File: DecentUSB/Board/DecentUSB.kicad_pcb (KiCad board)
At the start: 2 copper layers, 107 x 50.9 mm, 20 parts, among them J1 USB_A_Stacked, J2 Conn_01x28_Pin, J3 Conn_02x07_Counter_Clockwise, Q1 2N7000, Q2 2N7000, Q3 TP0610L, SW1 SW_Option, U1 Pico, U2 74LS245, U5 MCP23017_SP

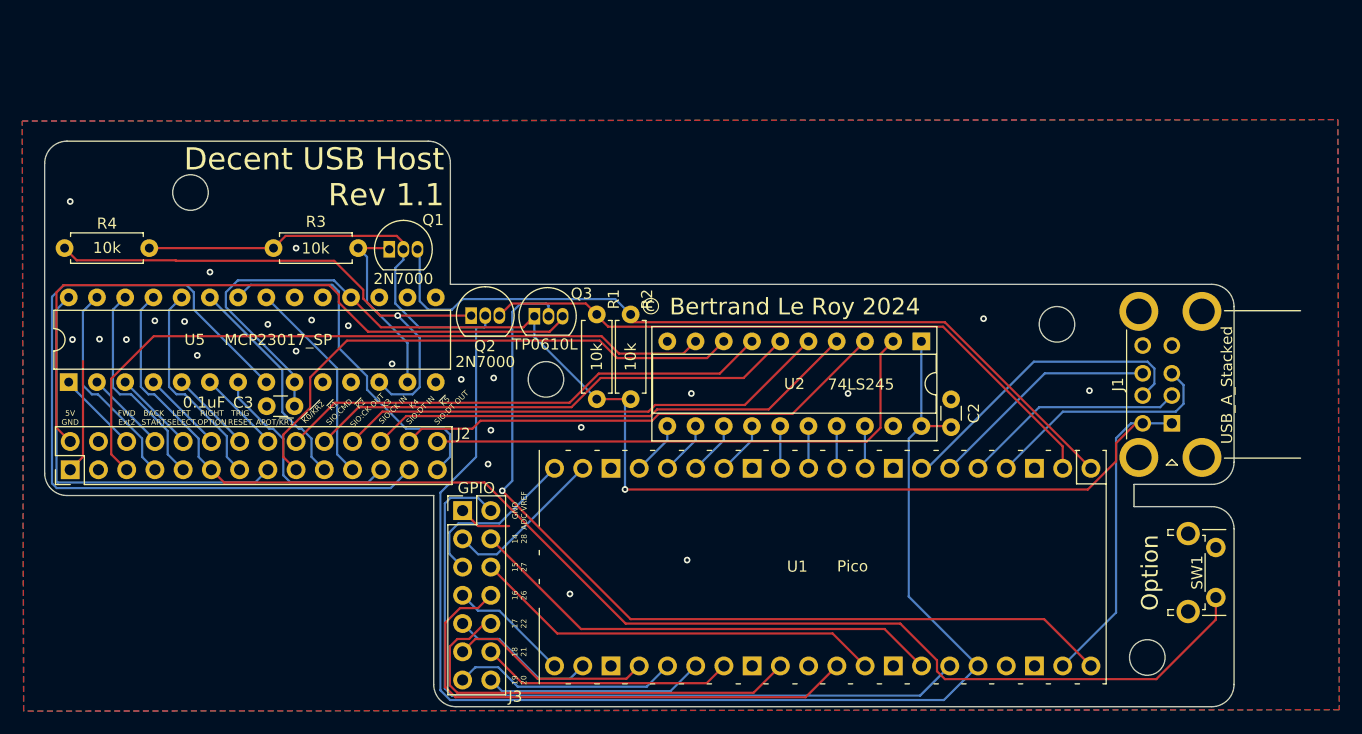
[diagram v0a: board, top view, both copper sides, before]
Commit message: DecentUSB Host board rev. 2
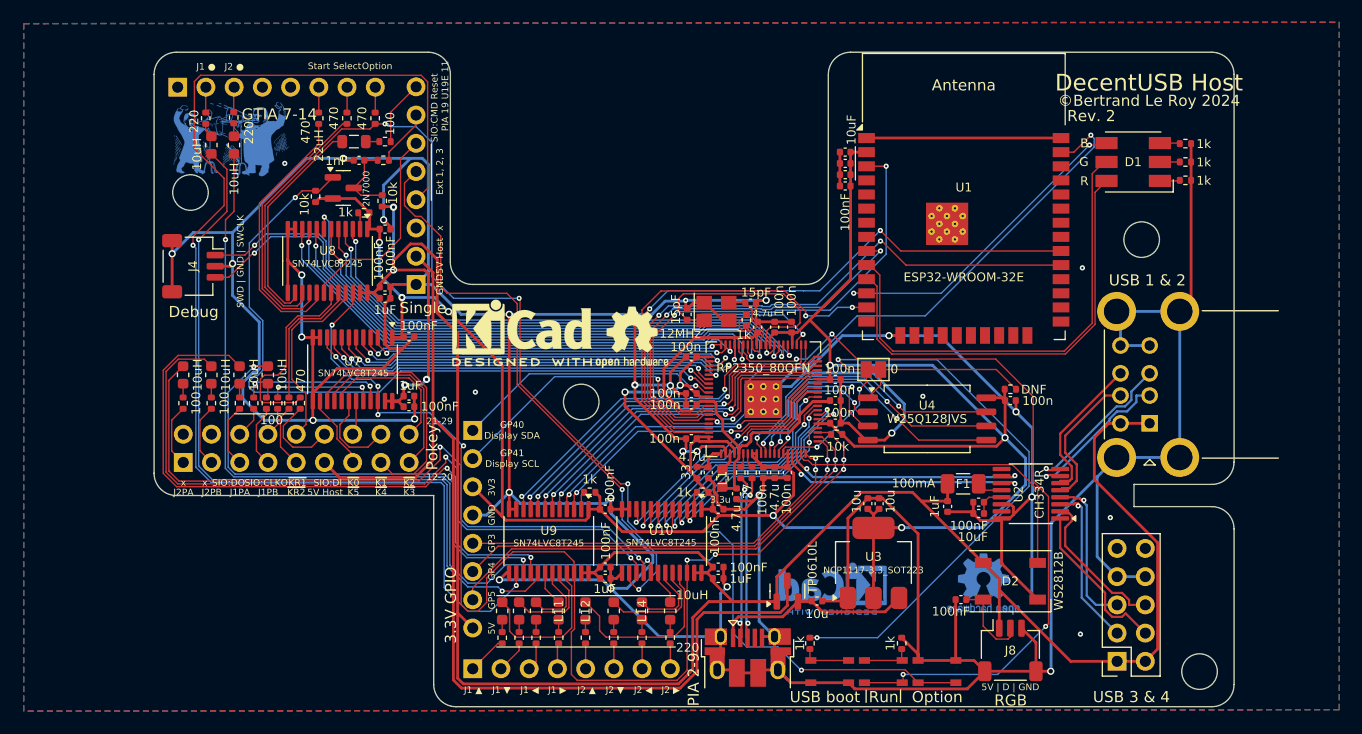
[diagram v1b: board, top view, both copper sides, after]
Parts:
- removed Q3: TP0610L, Package_TO_SOT_THT:TO-92L_Inline
- added C1: 100nF, Capacitor_SMD:C_0402_1005Metric, F.Cu at (138.4, 115.4)
- added C10: 100n, Capacitor_SMD:C_0402_1005Metric, F.Cu at (153.7, 93.9)
- added C11: 100n, Capacitor_SMD:C_0402_1005Metric, F.Cu at (146.2, 103.9)
- added C12: 100n, Capacitor_SMD:C_0402_1005Metric, F.Cu at (159.1, 102.5)
- added C13: 100n, Capacitor_SMD:C_0402_1005Metric, F.Cu at (154.8, 106.9)
- added C14: 100n, Capacitor_SMD:C_0402_1005Metric, F.Cu at (152.7, 106.9)
- added C15: 100n, Capacitor_SMD:C_0402_1005Metric, F.Cu at (155.2, 93.9)
- added C16: 100n, Capacitor_SMD:C_0402_1005Metric, F.Cu at (146.2, 96.5)
- added C17: 100n, Capacitor_SMD:C_0402_1005Metric, F.Cu at (146.2, 99.8)
- added C18: 4.7u, Capacitor_SMD:C_0402_1005Metric, F.Cu at (147.7, 106.9)
- added C19: 4.7u, Capacitor_SMD:C_0402_1005Metric, F.Cu at (153.7, 106.9)
- added C20: 4.7u, Capacitor_SMD:C_0402_1005Metric, F.Cu at (150.2, 108.8)
- added C21: 100n, Capacitor_SMD:C_0402_1005Metric, F.Cu at (174.9, 100.5)
- added C22: 10u, Capacitor_SMD:C_0402_1005Metric, F.Cu at (163.1, 109.7)
- added C23: 1nF, Capacitor_SMD:C_0402_1005Metric, F.Cu at (116.3, 78.8)
- added C24: 100nF, Capacitor_SMD:C_0402_1005Metric, F.Cu at (172.0, 109.6)
- added C25: 1uF, Capacitor_SMD:C_0402_1005Metric, F.Cu at (169.2, 110.0)
- added C26: 1uF, Capacitor_SMD:C_0402_1005Metric, F.Cu at (138.4, 116.5)
- added C27: 100nF, Capacitor_SMD:C_0402_1005Metric, F.Cu at (120.8, 101.0)
- added C28: 1uF, Capacitor_SMD:C_0402_1005Metric, F.Cu at (120.8, 100.1)
- added C29: 100nF, Capacitor_SMD:C_0402_1005Metric, F.Cu at (118.6, 90.2)
- added C30: 1uF, Capacitor_SMD:C_0402_1005Metric, F.Cu at (118.6, 91.3)
- added C31: 15pF, Capacitor_SMD:C_0402_1005Metric, F.Cu at (151.5, 91.7)
- added C32: 100nF, Capacitor_SMD:C_0402_1005Metric, F.Cu at (148.6, 115.4)
- added C33: 1uF, Capacitor_SMD:C_0402_1005Metric, F.Cu at (148.6, 116.5)
- added C34: 100nF, Capacitor_SMD:C_0402_1005Metric, F.Cu at (120.8, 94.7)
- added C35: 100nF, Capacitor_SMD:C_0402_1005Metric, F.Cu at (118.6, 85.0)
- added C36: 100nF, Capacitor_SMD:C_0402_1005Metric, F.Cu at (138.4, 110.2)
- added C37: 100nF, Capacitor_SMD:C_0402_1005Metric, F.Cu at (148.6, 110.2)
- added C38: 10uF, Capacitor_SMD:C_0402_1005Metric, F.Cu at (160.0, 78.1)
- added C39: 10uF, Capacitor_SMD:C_0402_1005Metric, F.Cu at (160.0, 79.1)
- added C4: 10u, Capacitor_SMD:C_0402_1005Metric, F.Cu at (157.5, 118.5)
- added C40: 10uF, Capacitor_SMD:C_0402_1005Metric, F.Cu at (160.0, 80.1)
- added C41: 100nF, Capacitor_SMD:C_0402_1005Metric, F.Cu at (160.0, 81.2)
- added C42: 100nF, Capacitor_SMD:C_0402_1005Metric, F.Cu at (170.4, 118.4)
- added C5: 10u, Capacitor_SMD:C_0402_1005Metric, F.Cu at (162.1, 109.7)
- added C6: 100n, Capacitor_SMD:C_0402_1005Metric, F.Cu at (146.2, 100.8)
- added C7: 4.7u, Capacitor_SMD:C_0402_1005Metric, F.Cu at (152.1, 93.9)
- added C8: 100n, Capacitor_SMD:C_0402_1005Metric, F.Cu at (159.1, 100.5)
- added C9: 100n, Capacitor_SMD:C_0402_1005Metric, F.Cu at (159.1, 98.6)
- added D1: LED_RGB, LED_SMD:LED_RGB_5050-6, F.Cu at (185.9, 79.0)
- added D2: WS2812B, LED_SMD:LED_WS2812B_PLCC4_5.0x5.0mm_P3.2mm, F.Cu at (174.9, 116.7)
- added F1: 100mA, Fuse:Fuse_1206_3216Metric, F.Cu at (170.6, 108.0)
- added G***: LOGO, Library:ScreamingAtTheRadio, B.Cu at (104.6, 75.9)
- added J1: USB_B_Micro, Connector_USB:USB_Micro-B_Amphenol_10103594-0001LF_Horizontal, F.Cu at (151.3, 123.6)
- added J4: SM03B-SRSS-TB, Connector_JST:JST_SH_SM03B-SRSS-TB_1x03-1MP_P1.00mm_Horizontal, F.Cu at (101.3, 88.4)
- added J5: Conn_02x09_Counter_Clockwise, Connector_PinSocket_2.54mm:PinSocket_2x09_P2.54mm_Vertical, F.Cu at (100.5, 103.5)
- added J6: Conn_02x05_Odd_Even, Connector_PinSocket_2.54mm:PinSocket_2x05_P2.54mm_Vertical, F.Cu at (184.5, 123.9)
- added J7: Conn_01x08, Connector_PinHeader_2.54mm:PinHeader_1x08_P2.54mm_Vertical, F.Cu at (126.5, 124.6)
- added J8: Conn_01x03, Connector_JST:JST_SH_SM03B-SRSS-TB_1x03-1MP_P1.00mm_Horizontal, F.Cu at (174.9, 122.9)
- added J9: Conn_01x08, Connector_PinHeader_2.54mm:PinHeader_1x08_P2.54mm_Vertical, F.Cu at (126.5, 103.1)
- added L1: 3.3u, Inductor_SMD:L_0603_1608Metric, F.Cu at (149.0, 107.4)
- added L10: 10uH, Inductor_SMD:L_0603_1608Metric, F.Cu at (132.2, 119.4)
- added L11: 10uH, Inductor_SMD:L_0603_1608Metric, F.Cu at (134.2, 119.4)
- added L12: 10uH, Inductor_SMD:L_0603_1608Metric, F.Cu at (136.7, 119.4)
- added L13: 10uH, Inductor_SMD:L_0603_1608Metric, F.Cu at (139.2, 119.4)
- added L14: 10uH, Inductor_SMD:L_0603_1608Metric, F.Cu at (141.7, 119.4)
- added L15: 10uH, Inductor_SMD:L_0603_1608Metric, F.Cu at (144.3, 119.4)
- added L16: 22uH, Inductor_SMD:L_0805_2012Metric, F.Cu at (115.8, 77.2)
- added L2: 10uH, Inductor_SMD:L_0603_1608Metric, F.Cu at (100.5, 98.2)
- added L3: 10uH, Inductor_SMD:L_0603_1608Metric, F.Cu at (103.0, 98.2)
- added L4: 10uH, Inductor_SMD:L_0603_1608Metric, F.Cu at (105.5, 98.2)
- added L5: 10uH, Inductor_SMD:L_0603_1608Metric, F.Cu at (108.1, 98.2)
- added L6: 10uH, Inductor_SMD:L_0603_1608Metric, F.Cu at (103.0, 77.5)
- added L7: 10uH, Inductor_SMD:L_0603_1608Metric, F.Cu at (105.0, 77.5)
- added L8: 10uH, Inductor_SMD:L_0603_1608Metric, F.Cu at (129.2, 119.4)
- added L9: 10uH, Inductor_SMD:L_0603_1608Metric, F.Cu at (130.7, 119.4)
- added R12: 10k, Resistor_SMD:R_0402_1005Metric, F.Cu at (112.4, 82.1)
- added R13: 10k, Resistor_SMD:R_0402_1005Metric, F.Cu at (118.4, 82.5)
- added R14: 100, Resistor_SMD:R_0402_1005Metric, F.Cu at (109.0, 100.7)
- added R15: 100, Resistor_SMD:R_0402_1005Metric, F.Cu at (106.8, 100.7)
- added R16: 100, Resistor_SMD:R_0402_1005Metric, F.Cu at (111.0, 100.7)
- added R17: 100, Resistor_SMD:R_0402_1005Metric, F.Cu at (100.5, 100.7)
- added R18: 100, Resistor_SMD:R_0402_1005Metric, F.Cu at (103.0, 100.7)
- added R19: 100, Resistor_SMD:R_0402_1005Metric, F.Cu at (105.5, 100.7)
- added R20: 100, Resistor_SMD:R_0402_1005Metric, F.Cu at (107.9, 100.7)
- added R21: 470, Resistor_SMD:R_0402_1005Metric, F.Cu at (110.0, 100.7)
- added R22: 220, Resistor_SMD:R_0402_1005Metric, F.Cu at (102.5, 75.1)
- added R23: 220, Resistor_SMD:R_0402_1005Metric, F.Cu at (105.0, 75.0)
- added R24: 470, Resistor_SMD:R_0402_1005Metric, F.Cu at (112.6, 75.1)
- added R25: 470, Resistor_SMD:R_0402_1005Metric, F.Cu at (115.2, 75.1)
- added R26: 470, Resistor_SMD:R_0402_1005Metric, F.Cu at (117.7, 75.1)
- added R27: 220, Resistor_SMD:R_0402_1005Metric, F.Cu at (129.2, 121.8)
- added R28: 220, Resistor_SMD:R_0402_1005Metric, F.Cu at (130.7, 121.8)
- added R29: 220, Resistor_SMD:R_0402_1005Metric, F.Cu at (132.2, 121.8)
- added R30: 220, Resistor_SMD:R_0402_1005Metric, F.Cu at (134.2, 121.8)
- added R31: 220, Resistor_SMD:R_0402_1005Metric, F.Cu at (136.7, 121.8)
- added R32: 220, Resistor_SMD:R_0402_1005Metric, F.Cu at (139.2, 121.8)
- added R33: 220, Resistor_SMD:R_0402_1005Metric, F.Cu at (141.7, 121.8)
- added R34: 220, Resistor_SMD:R_0402_1005Metric, F.Cu at (144.3, 121.8)
- added R35: 100, Resistor_SMD:R_0402_1005Metric, F.Cu at (118.6, 77.2)
- added R36: 10k, Resistor_SMD:R_0402_1005Metric, F.Cu at (159.3, 103.5)
- added R37: 1k, Resistor_SMD:R_0402_1005Metric, F.Cu at (116.7, 83.6)
- added R38: 1k, Resistor_SMD:R_0402_1005Metric, F.Cu at (137.0, 108.7)
- added R39: 1k, Resistor_SMD:R_0402_1005Metric, F.Cu at (147.2, 108.7)
- added R40: 1k, Resistor_SMD:R_0402_1005Metric, F.Cu at (190.6, 80.6)
- added R41: 1k, Resistor_SMD:R_0402_1005Metric, F.Cu at (190.6, 79.0)
- added R42: 1k, Resistor_SMD:R_0402_1005Metric, F.Cu at (190.6, 77.3)
- added R5: DNF, Resistor_SMD:R_0402_1005Metric, F.Cu at (174.9, 99.4)
- added R6: 100, Resistor_SMD:R_0402_1005Metric, F.Cu at (118.5, 78.8)
- added R7: 1k, Resistor_SMD:R_0402_1005Metric, F.Cu at (156.8, 122.3)
- added R8: 0, Jumper:SolderJumper-2_P1.3mm_Bridged_Pad1.0x1.5mm, F.Cu at (162.6, 97.7)
- added R9: 1k, Resistor_SMD:R_0402_1005Metric, F.Cu at (165.1, 122.3)
- added REF**: KiCad-Logo2_5mm_SilkScreen, Symbol:KiCad-Logo2_5mm_SilkScreen, F.Cu at (130.9, 94.4)
- added REF**: OSHW-Logo2_7.3x6mm_SilkScreen, Symbol:OSHW-Logo2_7.3x6mm_SilkScreen, F.Cu at (140.8, 94.8)
- added REF**: OSHW-Logo2_7.3x6mm_Copper, Symbol:OSHW-Logo2_7.3x6mm_Copper, B.Cu at (172.5, 117.0)
- added REF**: KiCad-Logo2_6mm_Copper, Symbol:KiCad-Logo2_6mm_Copper, B.Cu at (158.9, 116.7)
- added SW2: SW_USB_BOOT, DecenTKL:SW_Push_1P1T_XKB_TS-1177A-C, F.Cu at (158.6, 124.8)
- added SW3: SW_RUN, DecenTKL:SW_Push_1P1T_XKB_TS-1177A-C, F.Cu at (163.4, 124.8)
- added U10: SN74LVC8T245, Package_SO:TSSOP-24_4.4x7.8mm_P0.65mm, F.Cu at (143.5, 113.1)
- added U3: NCP1117-3.3_SOT223, Package_TO_SOT_SMD:SOT-223-3_TabPin2, F.Cu at (162.6, 115.1)
- added U4: W25Q128JVS, Package_SO:SOIC-8_7.5x5.85mm_P1.27mm, F.Cu at (167.4, 102.1)
- added U7: SN74LVC8T245, Package_SO:TSSOP-24_4.4x7.8mm_P0.65mm, F.Cu at (115.7, 97.6)
- added U8: SN74LVC8T245, Package_SO:TSSOP-24_4.4x7.8mm_P0.65mm, F.Cu at (113.4, 87.9)
- added U9: SN74LVC8T245, Package_SO:TSSOP-24_4.4x7.8mm_P0.65mm, F.Cu at (133.3, 113.1)
- added X4: 12MHz, Crystal:Crystal_SMD_Abracon_ABM8AIG-4Pin_3.2x2.5mm, F.Cu at (148.4, 92.4)
- C2: value 0.1uF -> 15pF; footprint Capacitor_THT:C_Disc_D3.0mm_W1.6mm_P2.50mm -> Capacitor_SMD:C_0402_1005Metric
- C3: value 0.1uF -> 10uF; footprint Capacitor_THT:C_Disc_D3.0mm_W1.6mm_P2.50mm -> Capacitor_SMD:C_0402_1005Metric
- J2: value Conn_01x28_Pin -> Conn_01x08; footprint Connector_PinHeader_2.54mm:PinHeader_2x14_P2.54mm_Vertical -> Connector_PinHeader_2.54mm:PinHeader_1x08_P2.54mm_Vertical
- J3: value Conn_02x07_Counter_Clockwise -> Conn_01x08; footprint Connector_PinHeader_2.54mm:PinHeader_2x07_P2.54mm_Vertical -> Connector_PinHeader_2.54mm:PinHeader_1x08_P2.54mm_Vertical
- Q1: footprint Package_TO_SOT_THT:TO-92_Inline -> Package_TO_SOT_SMD:SOT-23
- Q2: value 2N7000 -> TP0610L; footprint Package_TO_SOT_THT:TO-92_Inline -> Package_TO_SOT_SMD:SOT-23
- R1: value 10k -> 1k; footprint Resistor_THT:R_Axial_DIN0207_L6.3mm_D2.5mm_P7.62mm_Horizontal -> Resistor_SMD:R_0402_1005Metric
- R2: value 10k -> 33; footprint Resistor_THT:R_Axial_DIN0207_L6.3mm_D2.5mm_P7.62mm_Horizontal -> Resistor_SMD:R_0402_1005Metric
- R3, R4: value 10k -> 27; footprint Resistor_THT:R_Axial_DIN0207_L6.3mm_D2.5mm_P7.62mm_Horizontal -> Resistor_SMD:R_0402_1005Metric
- SW1: footprint Button_Switch_THT:SW_Tactile_SPST_Angled_PTS645Vx83-2LFS -> DecenTKL:SW_Push_1P1T_XKB_TS-1177A-C
- U1: value Pico -> ESP32-WROOM-32E; footprint Library:RPi_Pico_TH -> RF_Module:ESP32-WROOM-32D
- U2: value 74LS245 -> CH334R; footprint Package_DIP:DIP-20_W7.62mm_Socket -> Package_SO:QSOP-16_3.9x4.9mm_P0.635mm
- U5: value MCP23017_SP -> RP2350_80QFN; footprint Package_DIP:DIP-28_W7.62mm -> DecenTKL:RP2350-QFN-80-1EP_10x10_P0.4mm_EP3.4x3.4mm_ThermalVias
- USB1-2: renamed from J1; value USB_A_Stacked -> USB_A_Dual
- moved C3 64.8 mm to (172.0, 110.6), turned to 180 degrees
- moved U5 62.5 mm to (152.7, 100.3), turned to 180 degrees
- moved R4 56.9 mm to (150.6, 106.9), turned to 90 degrees
- moved R3 47.6 mm to (151.6, 106.9), turned to 90 degrees
- moved J3 45.9 mm to (100.0, 72.3), turned to 90 degrees
- moved Q2 37.7 mm to (154.8, 117.6), turned to 90 degrees
- moved J2 35.3 mm to (121.4, 90.0), turned to 180 degrees
- moved U1 32.9 mm to (170.7, 85.1), turned to 0 degrees
- moved SW1 27.5 mm to (168.3, 124.8), turned to 0 degrees
- moved C2 24.9 mm to (145.8, 92.7), turned to 90 degrees
- moved U2 16.9 mm to (176.7, 108.8), turned to 180 degrees
- moved R1 15.2 mm to (151.1, 93.2)
- moved REF** 10.8 mm to (186.7, 86.0)
- moved R2 8.90 mm to (146.7, 106.9)
- moved Q1 6.90 mm to (114.9, 81.3)
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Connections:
- C2 pad 1: GND -> /XIN
- C2 pad 2: 3.3V -> GND
- C3 pad 1: unconnected-(C3-Pad1) -> Net-(U2-VDD33)
- C3 pad 2: 5V -> GND
- J2 pad 2: unconnected-(J2-Pin_2-Pad2) -> +5V HOST
- J2 pad 3: EXT2 -> unconnected-(J2-Pin_3-Pad3)
- J2 pad 4: START -> EXT1
- J2 pad 5: SELECT -> EXT2
- J2 pad 6: OPTION -> EXT3
- J2 pad 7: RESET -> Net-(J2-Pin_7)
- J2 pad 8: ~{KR1} -> Net-(J2-Pin_8)
- J3 pad 1: GND -> unconnected-(J3-Pin_1-Pad1)
- J3 pad 2: GPIO14 -> Net-(J3-Pin_2)
- J3 pad 3: GPIO15 -> Net-(J3-Pin_3)
- J3 pad 4: GPIO16 -> unconnected-(J3-Pin_4-Pad4)
- J3 pad 5: GPIO17 -> unconnected-(J3-Pin_5-Pad5)
- J3 pad 6: GPIO18 -> Net-(J3-Pin_6)
- J3 pad 7: GPIO19 -> Net-(J3-Pin_7)
- J3 pad 8: GPIO20 -> Net-(J3-Pin_8)
- Q1 pad 1: Net-(Q1-S) -> GPIO39
- Q1 pad 2: 3.3V -> +3V3
- Q1 pad 3: Net-(Q1-D) -> SIO:COMMAND
- Q2 pad 1: Net-(Q2-S) -> +5V
- Q2 pad 2: 3.3V -> VBUS
- Q2 pad 3: Net-(Q2-D) -> +5V HOST
- R1 pad 1: 5V -> Net-(C31-Pad2)
- R1 pad 2: Net-(Q2-D) -> /XOUT
- R2 pad 1: 5V -> +3V3
- R2 pad 2: Net-(Q1-D) -> /VREG_AVDD
- R3 pad 1: 3.3V -> /USB_D+
- R3 pad 2: Net-(Q1-S) -> Net-(U5-USB_DP)
- R4 pad 1: 3.3V -> /USB_D-
- R4 pad 2: Net-(Q2-S) -> Net-(U5-USB_DM)
- U1 pad 1: Net-(Q1-D) -> GND
- U1 pad 10: Net-(U1-GPIO7) -> Net-(D1-GA)
- U1 pad 11: Net-(U1-GPIO8) -> Net-(D1-RA)
- U1 pad 12: Net-(U1-GPIO9) -> Net-(D1-BA)
- U1 pad 13: GND -> SPI1 TX
- U1 pad 14: Net-(U1-GPIO10) -> unconnected-(U1-IO12-Pad14)
- U1 pad 15: Net-(U1-GPIO11) -> GND
- U1 pad 16: Net-(U1-GPIO12) -> unconnected-(U1-IO13-Pad16)
- U1 pad 17: Net-(U1-GPIO13) -> unconnected-(U1-NC-Pad17)
- U1 pad 18: GND -> unconnected-(U1-NC-Pad18)
- U1 pad 19: GPIO14 -> unconnected-(U1-NC-Pad19)
- U1 pad 2: Net-(Q2-D) -> +3V3
- U1 pad 20: GPIO15 -> unconnected-(U1-NC-Pad20)
- U1 pad 21: GPIO16 -> unconnected-(U1-NC-Pad21)
- U1 pad 22: GPIO17 -> unconnected-(U1-NC-Pad22)
- U1 pad 23: GND -> unconnected-(U1-IO15-Pad23)
- U1 pad 24: GPIO18 -> unconnected-(U1-IO2-Pad24)
- U1 pad 25: GPIO19 -> unconnected-(U1-IO0-Pad25)
- U1 pad 26: GPIO20 -> unconnected-(U1-IO4-Pad26)
- U1 pad 27: GPIO21 -> unconnected-(U1-IO16-Pad27)
- U1 pad 28: GND -> unconnected-(U1-IO17-Pad28)
- U1 pad 29: GPIO22 -> SPI1 CSn
- U1 pad 3: GND -> GPIO42
- U1 pad 30: unconnected-(U1-RUN-Pad30) -> SPI1 SCK
- U1 pad 31: GPIO26 -> unconnected-(U1-IO19-Pad31)
- U1 pad 32: GPIO27 -> unconnected-(U1-NC-Pad32)
- U1 pad 33: GND -> unconnected-(U1-IO21-Pad33)
- U1 pad 34: GPIO28 -> unconnected-(U1-RXD0/IO3-Pad34)
- U1 pad 35: ADC_VREF -> unconnected-(U1-TXD0/IO1-Pad35)
- U1 pad 36: 3.3V -> unconnected-(U1-IO22-Pad36)
- U1 pad 37: unconnected-(U1-3V3_EN-Pad37) -> SPI1 RX
- U1 pad 39: 5V -> GND
- U1 pad 4: Net-(J1-D1+) -> unconnected-(U1-SENSOR_VP-Pad4)
- U1 pad 5: Net-(J1-D1-) -> unconnected-(U1-SENSOR_VN-Pad5)
- U1 pad 6: Net-(J1-D2+) -> unconnected-(U1-IO34-Pad6)
- U1 pad 7: Net-(J1-D2-) -> unconnected-(U1-IO35-Pad7)
- U1 pad 8: GND -> unconnected-(U1-IO32-Pad8)
- U1 pad 9: Net-(U1-GPIO6) -> GPIO43
- U2 pad 1: 3.3V -> /USB4-D-
- U2 pad 10: GND -> DMU-
- U2 pad 11: Net-(U1-GPIO13) -> DMU+
- U2 pad 12: Net-(U1-GPIO12) -> Net-(U2-V5)
- U2 pad 13: Net-(U1-GPIO11) -> Net-(U2-VDD33)
- U2 pad 14: Net-(U1-GPIO10) -> GND
- U2 pad 15: Net-(U1-GPIO9) -> unconnected-(U2-XO-Pad15)
- U2 pad 16: Net-(U1-GPIO8) -> GND
- U2 pad 2: ~{K5} -> /USB4-D+
- U2 pad 3: K4 -> /USB3-D-
- U2 pad 4: K3 -> /USB3-D+
- U2 pad 5: ~{K2} -> /USB2-D-
- U2 pad 6: ~{K1} -> /USB2-D+
- U2 pad 7: ~{K0} -> /USB1-D-
- U2 pad 8: ~{KR2} -> /USB1-D+
- U2 pad 9: EXT2 -> unconnected-(U2-~{RESET}/CDP-Pad9)
- U5 pad 1: J1:FWD -> GPIO4
- U5 pad 10: GND -> +1V1
- U5 pad 11: unconnected-(U5-NC-Pad11) -> GPIO12
- U5 pad 12: Net-(Q2-S) -> GPIO13
- U5 pad 13: Net-(Q1-S) -> GPIO14
- U5 pad 14: unconnected-(U5-NC-Pad14) -> GPIO15
- U5 pad 15: GND -> +3V3
- U5 pad 16: GND -> GPIO16
- U5 pad 17: GND -> GPIO17
- U5 pad 18: 5V -> GPIO18
- U5 pad 19: unconnected-(U5-INTB-Pad19) -> GPIO19
- U5 pad 2: J1:BACK -> GPIO5
- U5 pad 20: unconnected-(U5-INTA-Pad20) -> GPIO20
- U5 pad 21: SIO:CLOCK_OUT -> GPIO21
- U5 pad 22: SIO:DATA_OUT -> GPIO22
- U5 pad 23: SIO:COMMAND -> GPIO23
- U5 pad 24: RESET -> +3V3
- U5 pad 25: OPTION -> GPIO24
- U5 pad 26: SELECT -> GPIO25
- U5 pad 27: START -> GPIO26
- U5 pad 28: ~{KR1} -> GPIO27
- U5 pad 3: J1:LEFT -> GPIO6
- U5 pad 4: J1:RIGHT -> GPIO7
- U5 pad 5: J1:TRIGGER -> +3V3
- U5 pad 6: J1:A_POT -> GPIO8
- U5 pad 7: SIO:CLOCK_IN -> GPIO9
- U5 pad 8: SIO:DATA_IN -> GPIO10
- U5 pad 9: 5V -> GPIO11
- USB1-2 pad 1: 5V -> +5V
- USB1-2 pad 2: Net-(J1-D1-) -> /USB1-D-
- USB1-2 pad 3: Net-(J1-D1+) -> /USB1-D+
- USB1-2 pad 5: 5V -> +5V
- USB1-2 pad 6: Net-(J1-D2-) -> /USB2-D-
- USB1-2 pad 7: Net-(J1-D2+) -> /USB2-D+
- USB1-2 pad 9: unconnected-(J1-Shield-Pad9)_1 -> GND
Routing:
- net GND: track 15.0 -> 586.9 mm, vias 25 -> 34
- net +3V3: track 0.00 -> 241.1 mm, vias 0 -> 9
- net +5V: track 0.00 -> 213.8 mm, vias 0 -> 4
- net 3.3V: track 157.5 -> 0.00 mm
- net 5V: track 141.0 -> 0.00 mm, vias 1 -> 0
- net EXT1: track 0.00 -> 111.2 mm, vias 0 -> 2
- net GPIO6: track 0.00 -> 105.4 mm, vias 0 -> 8
- net +5V HOST: track 0.00 -> 92.6 mm
- net Net-(Q3-G): track 80.6 -> 0.00 mm, vias 1 -> 0
- net J2:TRIGGER: track 0.00 -> 77.2 mm, vias 0 -> 2
- net Net-(Q1-D): track 72.4 -> 0.00 mm
- net /RUN: track 0.00 -> 70.6 mm, vias 0 -> 4
- net ADC_VREF: track 68.3 -> 0.00 mm
- net GPIO39: track 0.00 -> 67.0 mm, vias 0 -> 2
- net J2:POTB: track 0.00 -> 65.4 mm, vias 0 -> 2
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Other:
- board size 107 x 50.9 mm -> 97.2 x 58.9 mm
- board text added: "12-20"
- board text added: "21-29"
- board text added: "3.3V GPIO"
- board text added: "3V3"
- board text added: "5V"
- board text added: "5V Host"
- board text added: "5V | D | GND"
- board text added: "B"
- board text added: "Debug"
- board text added: "DecentUSB Host"
- board text added: "Ext 1, 2, 3"
- board text added: "G"
- board text added: "GND"
- board text added: "GP3"
- board text added: "GP4"
- board text added: "GP40 Display SDA"
- board text added: "GP41 Display SCL"
- board text added: "GP5"
- board text added: "GTIA 7-14"
- board text added: "J1 ▲"
- board text added: "J1 ▶"
- board text added: "J1 ▼"
- board text added: "J1 ◀"
- board text added: "J1 ●"
- board text added: "J1PA"
- board text added: "J1PB"
- board text added: "J2 ▲"
- board text added: "J2 ▶"
- board text added: "J2 ▼"
- board text added: "J2 ◀"
- board text added: "J2 ●"
- board text added: "J2PA"
- board text added: "J2PB"
- board text added: "PIA 2-9"
- board text added: "Pokey"
- board text added: "R"
- board text added: "RGB"
- board text added: "Reset U19E 11"
- board text added: "Rev. 2"
- board text added: "Run"
- board text added: "SIO:CLKO"
- board text added: "SIO:CMD PIA 19"
- board text added: "SIO:DI"
- board text added: "SIO:DO"
- board text added: "SWD | GND | SWCLK"
- board text added: "Select"
- board text added: "Single"
- board text added: "Start"
- board text added: "USB 1 & 2"
- board text added: "USB 3 & 4"
- board text added: "USB boot"
- board text added: "x"
- board text added: "~{K0}"
- board text added: "~{K1}"
- board text added: "~{K2}"
- board text added: "~{K3}"
- board text added: "~{K4}"
- board text added: "~{K5}"
- board text added: "~{KR1}"
- board text added: "~{KR2}"
- board text added: "©Bertrand Le Roy 2024"
- board text removed: "14 28"
- board text removed: "15 27"
- board text removed: "16 26"
- board text removed: "17 22"
- board text removed: "18 21"
- board text removed: "19 20"
- board text removed: "5V GND"
- board text removed: "APOT/~{KR1}"
- board text removed: "BACK START"
- board text removed: "Decent USB Host"
- board text removed: "Decent USB Host Rev 1.1"
- board text removed: "FWD Ext2"
- board text removed: "GND ADC VREF"
- board text removed: "GPIO"
- board text removed: "K3 SIO:CK IN"
- board text removed: "K4 SIO:DT IN"
- board text removed: "LEFT SELECT"
- board text removed: "RIGHT OPTION"
- board text removed: "TRIG RESET"
- board text removed: "~{K0}/~{KR2}"
- board text removed: "~{K1} SIO:CMD"
- board text removed: "~{K2} SIO:CK OUT"
- board text removed: "~{K5} SIO:DT OUT"
